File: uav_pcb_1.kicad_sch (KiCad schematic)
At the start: 45 parts, among them J1 USB_B_Micro, J2 Conn_02x08_Odd_Even, U1 STM32F405RGTx, U10 CH330N, U4 SN74LVC1G04DCKR, U5 PCA9685BS, U8 LD39200PU33R, U9 USBLC6-2SC6, Y1 Crystal_GND24

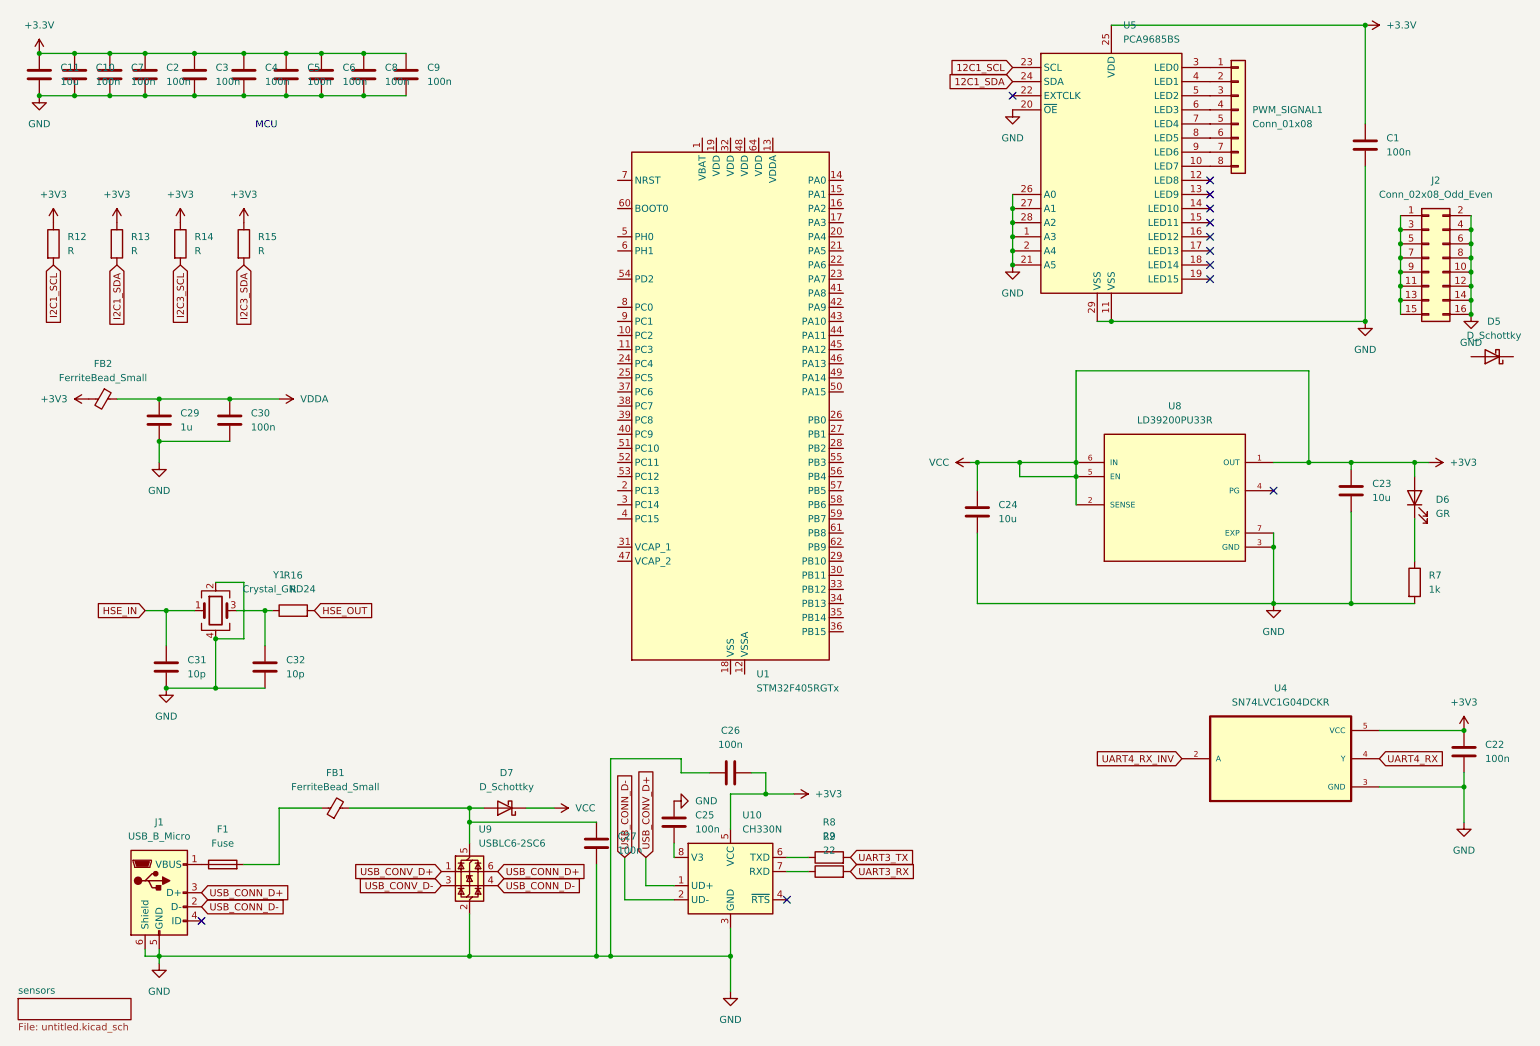
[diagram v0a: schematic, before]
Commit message: Add files via upload
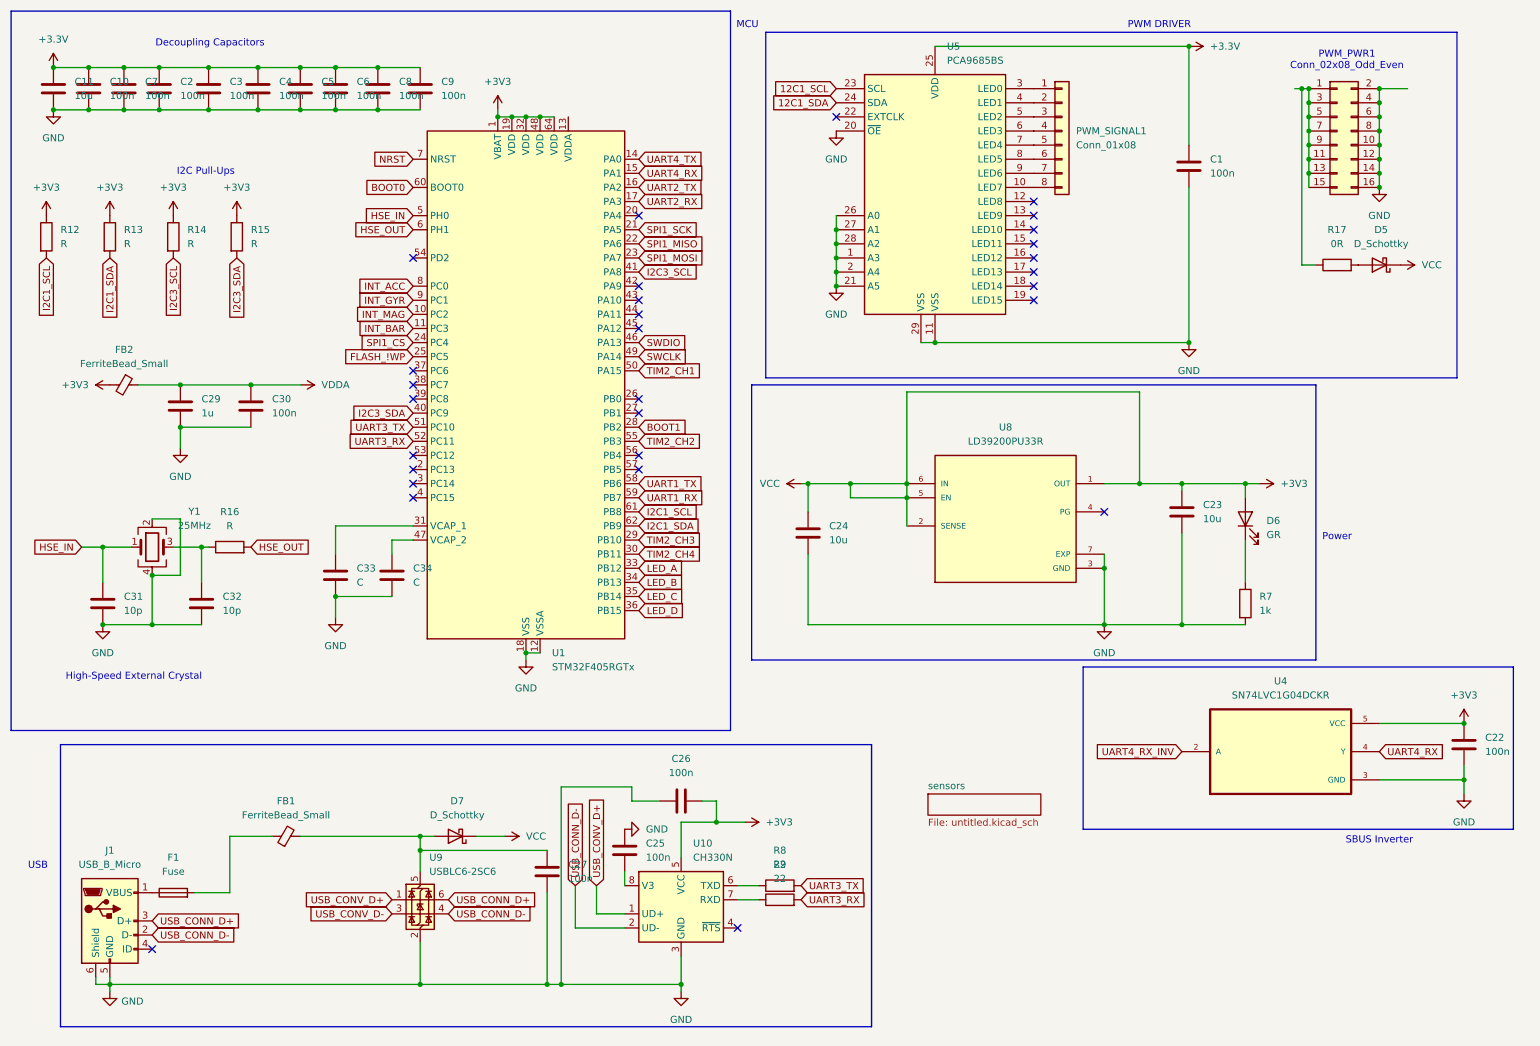
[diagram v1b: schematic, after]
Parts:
- added C33, C34: C, symbol Device:C
- added R17: 0R, symbol Device:R
- Y1: value Crystal_GND24 -> 25MHz
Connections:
- net +3V3: now also D5.1 (K), U1.1 (VBAT), U1.19 (VDD), U1.32 (VDD), U1.48 (VDD), U1.64 (VDD)
- net GND: now also U1.12 (VSSA), U1.18 (VSS), U1.63 (VSS), C33.2, C34.2
- net HSE_IN: now also U1.5 (PH0)
- net HSE_OUT: now also U1.6 (PH1)
- net I2C1_SCL: now also U1.61 (PB8)
- net I2C1_SDA: now also U1.62 (PB9)
- net I2C3_SCL: now also U1.41 (PA8)
- net I2C3_SDA: now also U1.40 (PC9)
- net UART3_RX: now also U1.52 (PC11)
- net UART3_TX: now also U1.51 (PC10)
- net UART4_RX: now also U1.15 (PA1)
- net INT_MAG: now reaches U1.10 (PC2)
- net INT_BAR: now reaches U1.11 (PC3)
- net UART4_TX: now reaches U1.14 (PA0)
- net UART2_TX: now reaches U1.16 (PA2)
- net UART2_RX: now reaches U1.17 (PA3)
- net SPI1_SCK: now reaches U1.21 (PA5)
- net SPI1_MISO: now reaches U1.22 (PA6)
- net SPI1_MOSI: now reaches U1.23 (PA7)
- net SPI1_CS: now reaches U1.24 (PC4)
- net FLASH_!WP: now reaches U1.25 (PC5)
- net BOOT1: now reaches U1.28 (PB2)
- net TIM2_CH3: now reaches U1.29 (PB10)
- net TIM2_CH4: now reaches U1.30 (PB11)
- net at U1.31 (VCAP_1): now also C33.1
- net LED_A: now reaches U1.33 (PB12)
- net LED_B: now reaches U1.34 (PB13)
- net LED_C: now reaches U1.35 (PB14)
- net LED_D: now reaches U1.36 (PB15)
- net SWDIO: now reaches U1.46 (PA13)
- net at U1.47 (VCAP_2): now also C34.1
- net SWCLK: now reaches U1.49 (PA14)
- net TIM2_CH1: now reaches U1.50 (PA15)
- net TIM2_CH2: now reaches U1.55 (PB3)
- net UART1_TX: now reaches U1.58 (PB6)
- net UART1_RX: now reaches U1.59 (PB7)
- net BOOT0: now reaches U1.60 (BOOT0)
- net NRST: now reaches U1.7 (NRST)
- net INT_ACC: now reaches U1.8 (PC0)
- net INT_GYR: now reaches U1.9 (PC1)
- net at J2.1 (Pin_1), J2.11 (Pin_11), J2.13 (Pin_13)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: now also R17.1
- net at D5.2 (A): now also R17.2
- no-connect marks 12 -> 29
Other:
- note added: "Decoupling Capacitors"
- note added: "High-Speed External Crystal"
- note added: "I2C Pull-Ups"
- note added: "PWM DRIVER"
- note added: "PWM_PWR1 Conn_02x08_Odd_Even"
- note added: "Power"
- note added: "SBUS Inverter"
- note added: "USB"
- moved on the sheet: C1, C10, C11, C2, C22, C23, C24, C25, C26, C27, C29, C3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
